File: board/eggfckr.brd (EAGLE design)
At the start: 53.6 x 21.6 mm, 8 parts, among them U1 ATTINY85-20PU

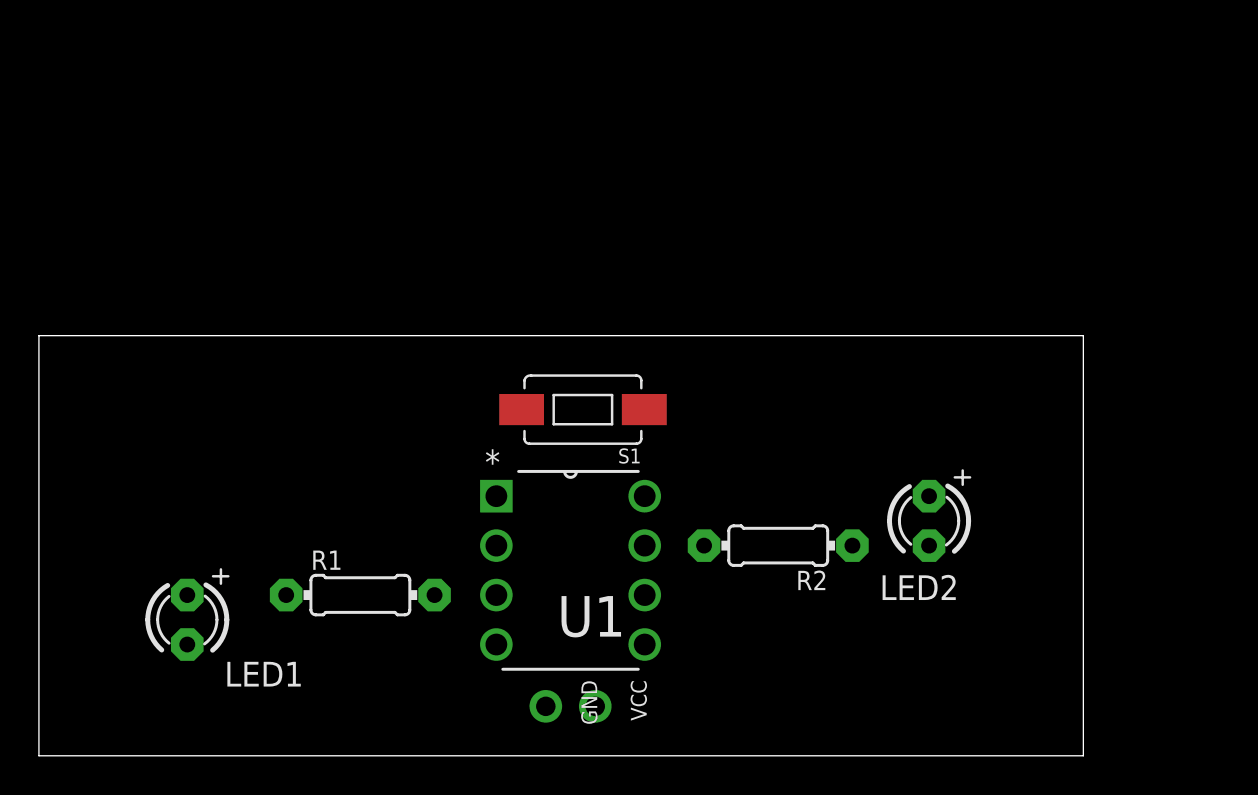
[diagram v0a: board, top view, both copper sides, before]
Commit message: whats going on'
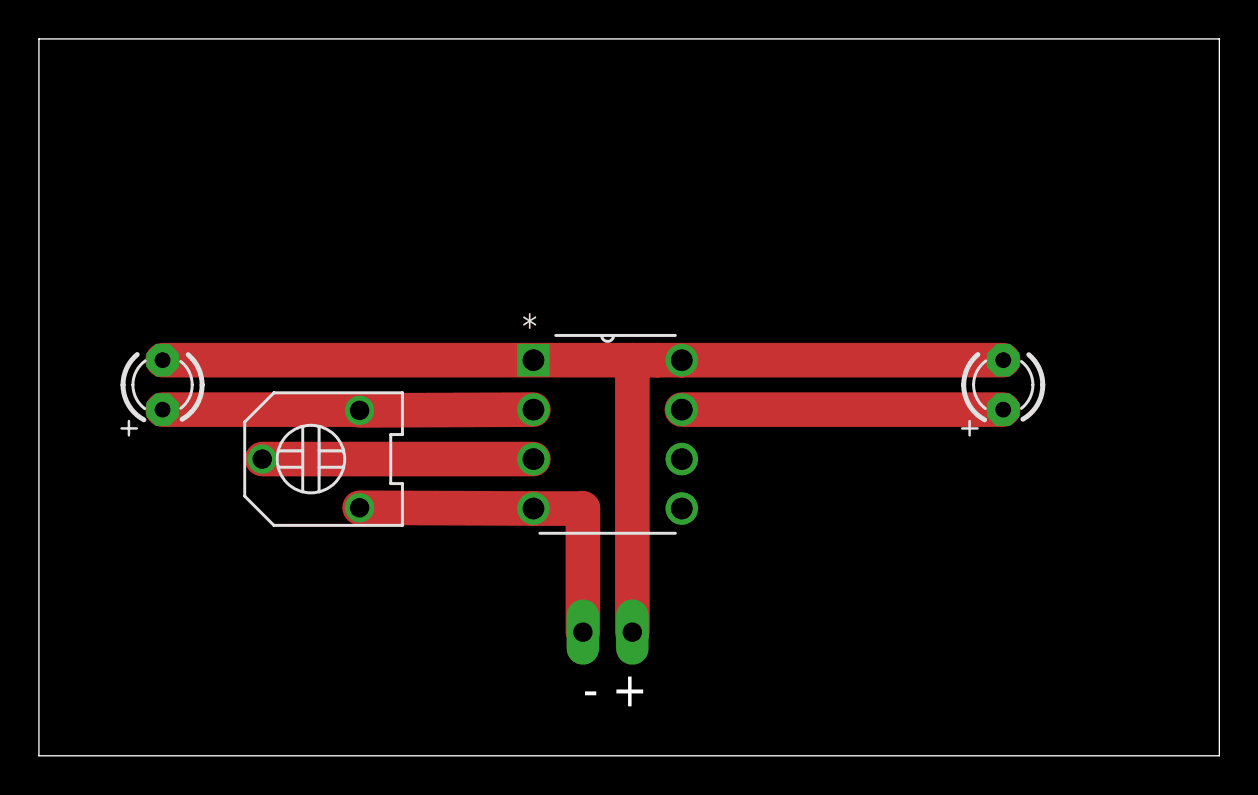
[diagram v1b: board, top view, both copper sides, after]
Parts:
- removed GND, VCC: (no value), microbuilder:1X01_ROUND
- removed R1, R2: (no value), adafruit:0204/7
- removed S1: SWITCH-MOMENTARY-2-SMD-1101NE, ATtami:TACTILE-SWITCH-1101NE
- removed U1: ATTINY85-20PU, Atmel_By_element14_Batch_1-00:DIP254P762X533-8
- added +, -: (no value), eggfckr:1X01_OVAL
- added ATINY85: ATTINY85-20PU, eggfckr:DIP254P762X533-8
- added R3: (no value), eggfckr:TRIMMER_3306F
- moved LED1 12.1 mm to (6.35, 19.1), turned to 90 degrees
- moved LED2 7.96 mm to (49.5, 19.1), turned to 90 degrees
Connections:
- removed net N$4: S1.P$2, U1.1
- removed net N$5: S1.P$1, U1.2
- removed net N$7: LED2.K, R2.1
- net GND: now also -.1, ATINY85.4, R3.1; no longer GND.1, LED1.K, U1.4
- net N$1: now also ATINY85.7, LED2.A; no longer R2.2, U1.7
- net N$2: now also ATINY85.3, R3.2; no longer R1.2, U1.3
- net N$3: now also ATINY85.2, LED1.K; no longer LED1.A, R1.1
- net VCC: now also +.1, ATINY85.8, LED1.A, LED2.K, R3.3; no longer LED2.A, U1.8, VCC.1
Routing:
- net VCC: track 0.00 -> 50.9 mm
- net N$3: track 0.00 -> 25.4 mm
- net GND: track 0.00 -> 17.8 mm
- net N$1: track 0.00 -> 16.5 mm
- net N$2: track 0.00 -> 13.9 mm
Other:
- board size 53.6 x 21.6 mm -> 60.6 x 36.8 mm
- board text added: "- +"
